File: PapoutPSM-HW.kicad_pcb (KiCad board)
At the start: 4 copper layers, 57 x 45 mm, 75 parts, among them J1 53015-0510, J2 53015-0510, Q1 NTK3134NT1G, Q2 NTK3134NT1G, Q3 NTK3134NT1G, U1 STM32G030F6, U2 SP3232EEY-L, U3 74HC4049, U4 TPS5430DDA, U5 RT8259GJ6

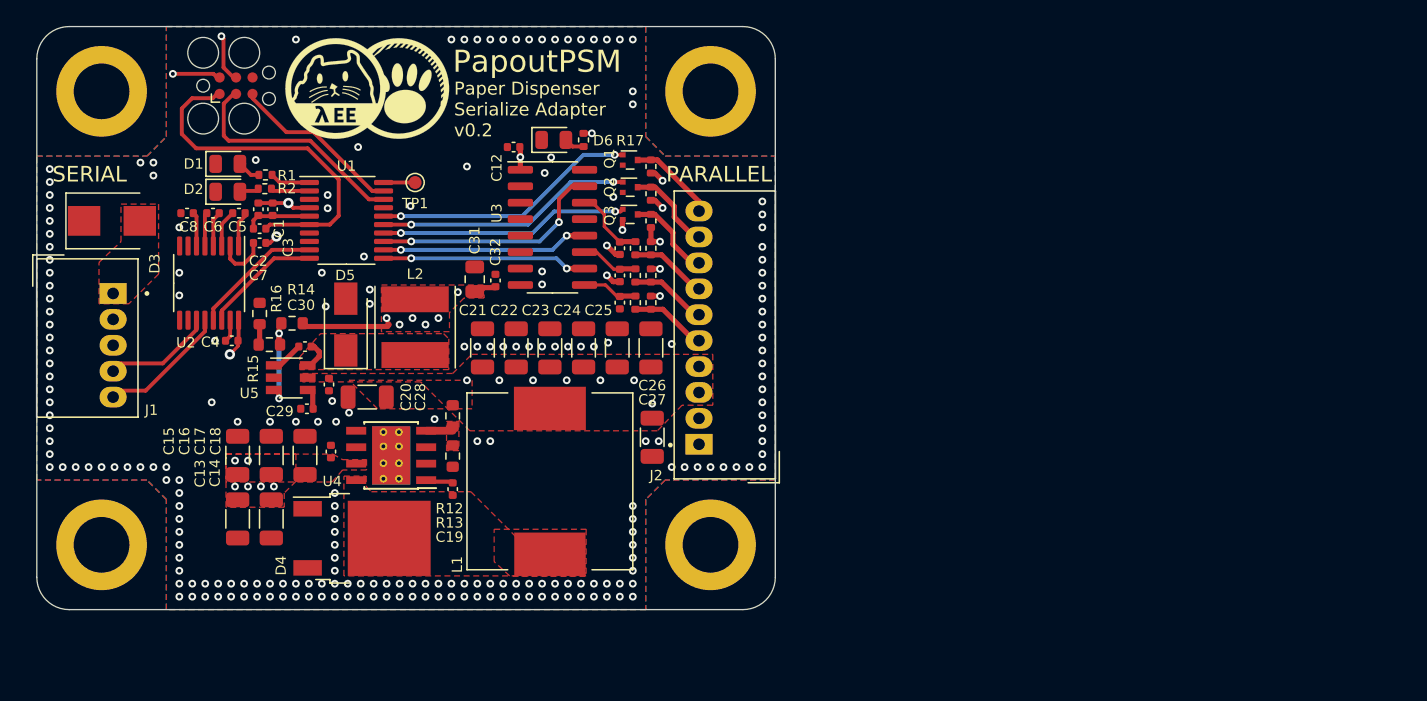
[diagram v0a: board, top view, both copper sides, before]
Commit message: release/v3 update
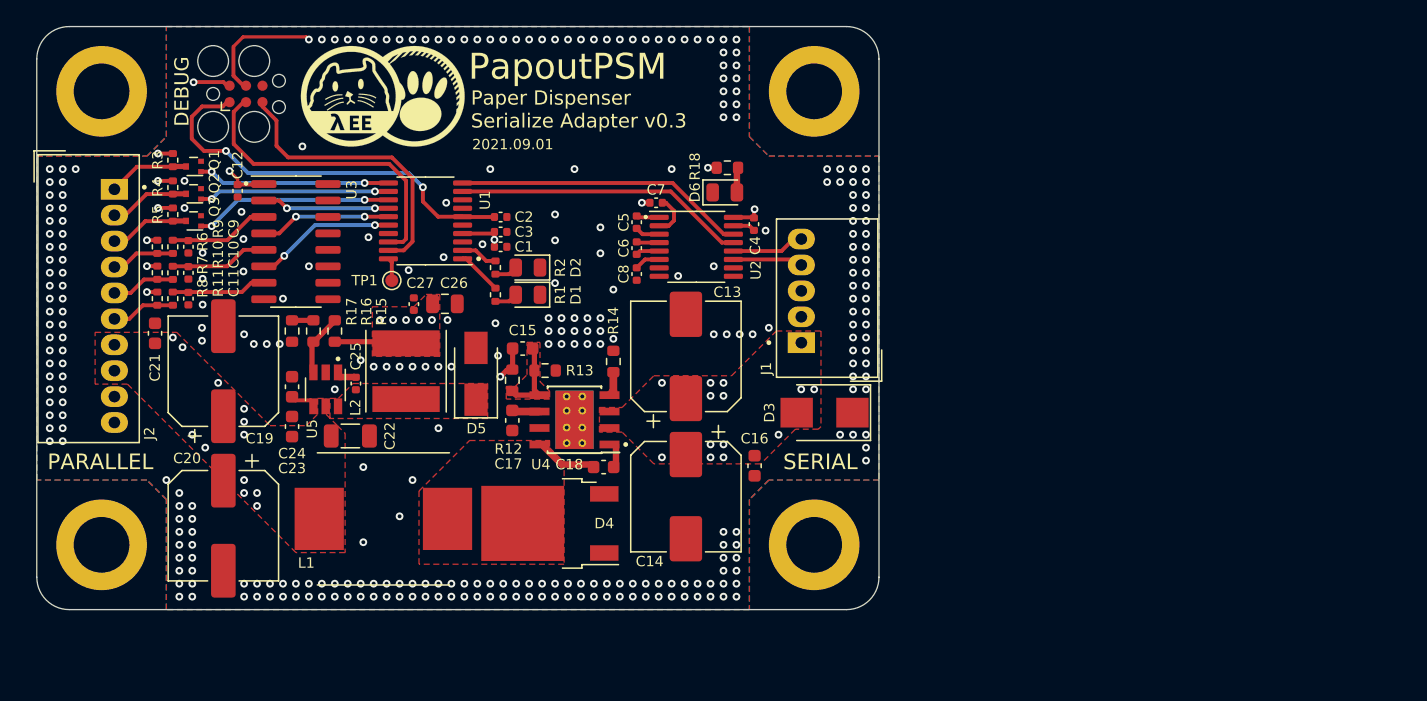
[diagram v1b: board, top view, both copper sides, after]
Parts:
- removed the C16 at (38.1, 83.1)
- removed the C22 at (57.0, 74.8)
- removed the C23 at (59.6, 74.8)
- removed the C24 at (62.2, 74.8)
- removed the C25 at (64.8, 74.8)
- removed the C26 at (67.4, 74.8)
- removed the C27 at (67.5, 81.7)
- added C19: 100uF, Capacitor_SMD:CP_Elec_8x6.9, F.Cu at (34.4, 76.6)
- added C20: 100uF, Capacitor_SMD:CP_Elec_8x6.9, F.Cu at (34.4, 88.5)
- added R14: 20k, Resistor_SMD:R_0603_1608Metric, F.Cu at (64.5, 75.8)
- C13, C14: value 10uF 50V -> 68uF; footprint Capacitor_SMD:C_1206_3216Metric -> Capacitor_SMD:CP_Elec_8x10
- C15: value 10uF 50V -> 330pF; footprint Capacitor_SMD:C_1206_3216Metric -> Capacitor_SMD:C_0603_1608Metric
- C16: renamed from C18; value 100nF -> 100nF 50V; footprint Capacitor_SMD:C_0402_1005Metric -> Capacitor_SMD:C_0603_1608Metric
- C17: value 10uF 50V -> 22nF; footprint Capacitor_SMD:C_1206_3216Metric -> Capacitor_SMD:C_0603_1608Metric
- C18: renamed from C19; value 10nF -> 100nF 50V; footprint Capacitor_SMD:C_0402_1005Metric -> Capacitor_SMD:C_0603_1608Metric
- C21: value 10uF 50V -> 100nF 50V; footprint Capacitor_SMD:C_1206_3216Metric -> Capacitor_SMD:C_0603_1608Metric
- C23: renamed from C20; value 100nF -> 100nF 50V; footprint Capacitor_SMD:C_0402_1005Metric -> Capacitor_SMD:C_0603_1608Metric
- C24: renamed from C29; value 100nF -> 100nF 50V; footprint Capacitor_SMD:C_0402_1005Metric -> Capacitor_SMD:C_0603_1608Metric
- D4: value MBRD20200CT-13 -> MBRD20150CT-13
- L1: value MWSA1206S-330MT -> SPM10040T-4R7M; footprint Power_Inductor_Extended:L_Sunlord-MWSA1206S -> TDK-SPM10040:L_TDK_SPM10040
- R12: renamed from R13; value 1.13k -> 150k
- R13: renamed from R12; value 10k -> 10k 0.1W
- R18: renamed from R17; value 4.7k -> 10k 0.1W; footprint Resistor_SMD:R_0402_1005Metric -> Resistor_SMD:R_0603_1608Metric
- R3, R4, R5: value 4.7k -> 8.2k
- R6, R7, R8: value 4.7k -> 27k
- U1: value STM32G030F6 -> STM32G031F8P6
- U4: value TPS5430DDA -> LMR14050SDDA
- moved H2 65.2 mm to (80.0, 90.0), turned to 90 degrees
- moved H4 65.2 mm to (80.0, 55.0), turned to 90 degrees
- moved H1 58.6 mm to (25.0, 90.0), turned to 90 degrees
- moved H3 58.6 mm to (25.0, 55.0), turned to 90 degrees
- moved D3 57.0 mm to (80.8, 79.8), turned to 180 degrees
- moved J1 53.3 mm to (79.0, 74.4), turned to 90 degrees
- moved J2 49.2 mm to (26.0, 62.6), turned to -90 degrees
- moved C4 41.3 mm to (75.3, 65.2), turned to -90 degrees
- moved R8 38.1 mm to (29.3, 71.0)
- moved R7 38.1 mm to (29.3, 69.0)
- moved R6 38.1 mm to (29.3, 67.0)
- moved U2 37.7 mm to (70.9, 67.0), turned to 0 degrees
- moved R3 36.9 mm to (30.5, 60.3), turned to 90 degrees
- moved R5 36.9 mm to (30.5, 64.5), turned to 90 degrees
- moved R4 36.9 mm to (30.5, 62.4), turned to 90 degrees
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- renumbered C28 to C22, C30 to C25, C31 to C26, C32 to C27, R14 to R15, R15 to R16, R16 to R17
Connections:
- net /Power/BIG_PH renamed /Power/BIG_SW
- net Net-(C19-Pad1) renamed /Power/BIG_BOOT
- C15 pad 1: +24V -> +12V
- C15 pad 2: GND -> /Power/BIG_FB
- C17 pad 1: +24V -> /Power/BIG_SS
- J2 pad 1: GND -> /Parallel_IO/J_INHIBIT
- J2 pad 10: /Parallel_IO/J_INHIBIT -> GND
- J2 pad 2: GND -> /Parallel_IO/J_RESET
- J2 pad 3: +12V -> /Parallel_IO/J_PULSE
- J2 pad 4: +12V -> /Parallel_IO/J_OUT_PULSE
- J2 pad 5: /Parallel_IO/J_ERROR -> /Parallel_IO/J_EMPTY
- J2 pad 6: /Parallel_IO/J_EMPTY -> /Parallel_IO/J_ERROR
- J2 pad 7: /Parallel_IO/J_OUT_PULSE -> +12V
- J2 pad 8: /Parallel_IO/J_PULSE -> +12V
- J2 pad 9: /Parallel_IO/J_RESET -> GND
- R12 pad 1: /Power/BIG_VS -> +12V
- R12 pad 2: GND -> /Power/BIG_FB
- R13 pad 1: +12V -> /Power/BIG_FB
- R13 pad 2: /Power/BIG_VS -> GND
- U1 pad 11: /P_ERROR -> /P_INHIBIT
- U1 pad 12: /P_EMPTY -> /P_RESET
- U1 pad 13: /P_OUT_PULSE -> /P_PULSE
- U1 pad 14: /P_PULSE -> /P_OUT_PULSE
- U1 pad 15: /P_RESET -> /P_EMPTY
- U1 pad 16: /P_INHIBIT -> /P_ERROR
- U3 pad 10: /P_ERROR -> unconnected-(U3-Pad10)
- U3 pad 11: Net-(C10-Pad1) -> GND
- U3 pad 12: /P_EMPTY -> unconnected-(U3-Pad12)
- U3 pad 14: Net-(C9-Pad1) -> GND
- U3 pad 15: /P_OUT_PULSE -> unconnected-(U3-Pad15)
- U3 pad 2: unconnected-(U3-Pad2) -> /P_OUT_PULSE
- U3 pad 3: GND -> Net-(C9-Pad1)
- U3 pad 4: unconnected-(U3-Pad4) -> /P_EMPTY
- U3 pad 5: GND -> Net-(C10-Pad1)
- U3 pad 6: unconnected-(U3-Pad6) -> /P_ERROR
- U3 pad 7: GND -> Net-(C11-Pad1)
- U3 pad 9: Net-(C11-Pad1) -> GND
- U4 pad 2: unconnected-(U4-Pad2) -> +24V
- U4 pad 3: unconnected-(U4-Pad3) -> +24V
- U4 pad 4: /Power/BIG_VS -> /Power/BIG_RTS
- U4 pad 5: unconnected-(U4-Pad5) -> /Power/BIG_FB
- U4 pad 6: GND -> /Power/BIG_SS
- U4 pad 7: +24V -> GND
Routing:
- net /M_RX: track 9.17 -> 22.5 mm
- net /M_TX: track 10.2 -> 22.5 mm
- net /SWCLK: track 13.6 -> 22.5 mm
- net /P_OUT_PULSE: track 18.3 -> 10.2 mm
- net /SWDIO: track 17.9 -> 24.0 mm
- net /Power/BIG_FB: track 0.00 -> 5.97 mm
- net /P_EMPTY: track 16.0 -> 10.4 mm
- net /P_INHIBIT: track 20.4 -> 15.1 mm
- net /Power/BIG_SW: track 0.00 -> 4.90 mm
- net /P_RESET: track 19.8 -> 15.0 mm
- net /P_ERROR: track 15.8 -> 11.2 mm
- net /R_RXD: track 10.0 -> 5.63 mm
- net +3V3: track 23.1 -> 19.0 mm, vias 12 -> 11
- net /NRST: track 27.5 -> 31.4 mm, vias 0 -> 2
- net /P_PULSE: track 19.2 -> 15.6 mm
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- added copper zone on F.Cu, net /Power/BIG_FB
- removed copper zone on F.Cu, net /Power/BIG_VS
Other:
- board size 57 x 45 mm -> 65 x 45 mm
- board text added: "2021.09.01"
- board text added: "DEBUG"
- board text added: "Paper Dispenser Serialize Adapter v0.3"
- board text added: "github.com/pmnxis/PapoutPSM-HW CERN-OHL-S-2.0"
- board text removed: "Paper Dispenser Serialize Adapter v0.2"
- board text removed: "github.com/PapoutPSM-HW CERN-OHL-S-2.0"

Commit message: before release v0.5
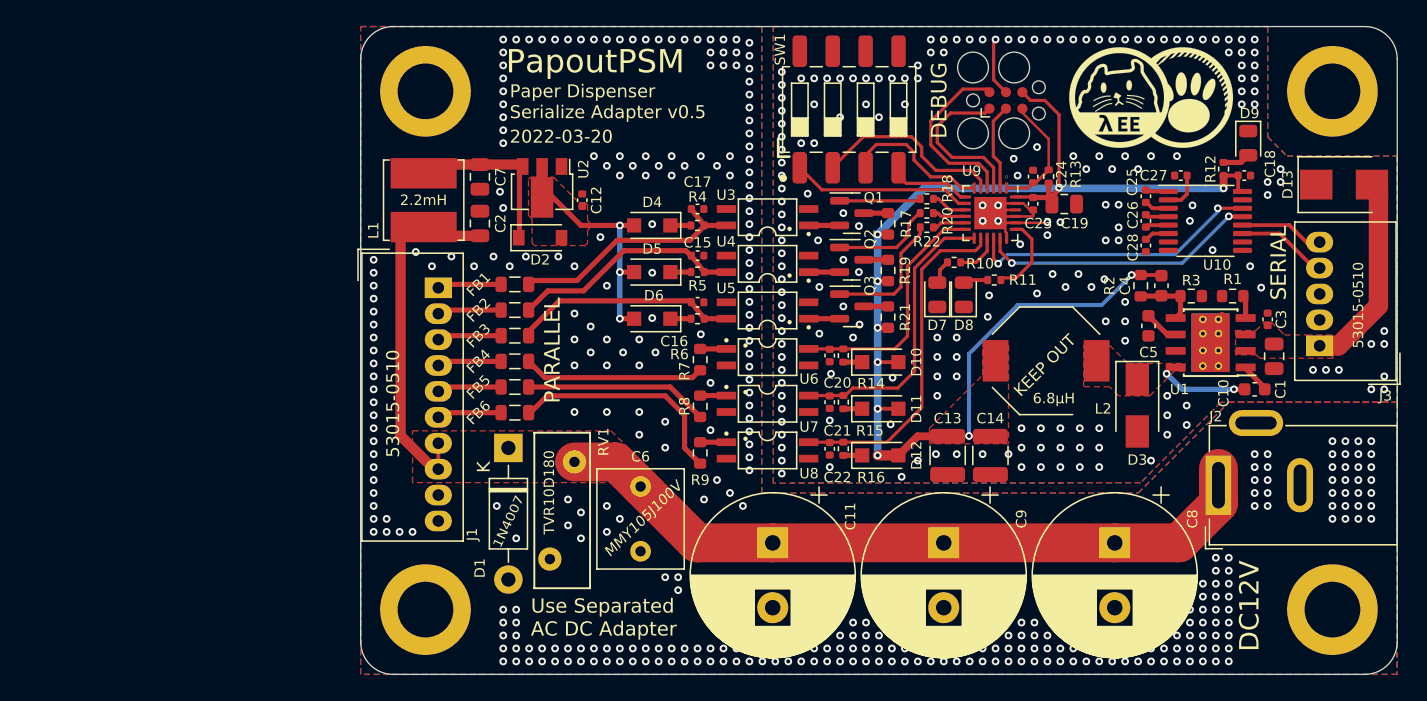
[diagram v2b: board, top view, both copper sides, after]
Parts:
- removed TP1: TestPoint, TestPoint:TestPoint_Pad_D1.0mm
- added C28: 100nF, Capacitor_SMD:C_0402_1005Metric, F.Cu at (105.6, 66.9)
- added D10: 1N4007, Diode_SMD:D_SOD-123F, F.Cu at (85.1, 75.9)
- added D11: 1N4007, Diode_SMD:D_SOD-123F, F.Cu at (85.1, 79.5)
- added D12: 1N4007, Diode_SMD:D_SOD-123F, F.Cu at (85.1, 83.1)
- added D13: SMBJ28CA, Diode_SMD:D_SMB, F.Cu at (120.9, 62.2)
- added D7: LED_YELLOW, LED_SMD:LED_0805_2012Metric, F.Cu at (89.5, 70.7)
- added D8: LED_YELLOW, LED_SMD:LED_0805_2012Metric, F.Cu at (91.5, 70.7)
- added D9: LED GREEN, LED_SMD:LED_0805_2012Metric, F.Cu at (113.5, 59.0)
- added FB1: GZ2012D601TF, Inductor_SMD:L_0805_2012Metric, F.Cu at (56.9, 69.9)
- added FB2: GZ2012D601TF, Inductor_SMD:L_0805_2012Metric, F.Cu at (56.9, 71.9)
- added FB3: GZ2012D601TF, Inductor_SMD:L_0805_2012Metric, F.Cu at (56.9, 73.9)
- added FB4: GZ2012D601TF, Inductor_SMD:L_0805_2012Metric, F.Cu at (56.9, 75.8)
- added FB5: GZ2012D601TF, Inductor_SMD:L_0805_2012Metric, F.Cu at (56.9, 77.8)
- added FB6: GZ2012D601TF, Inductor_SMD:L_0805_2012Metric, F.Cu at (56.9, 79.8)
- added J3: 53015-0510, Molex-53015:Molex_MicroBlade_53015-0500_1x05_P2.00mm_Right, F.Cu at (119.0, 74.6)
- added R19: 660, Resistor_SMD:R_0603_1608Metric, F.Cu at (85.7, 68.8)
- added R20: 4.7k, Resistor_SMD:R_0402_1005Metric, F.Cu at (88.7, 64.4)
- added R21: 660, Resistor_SMD:R_0603_1608Metric, F.Cu at (85.7, 72.4)
- added R22: 4.7k, Resistor_SMD:R_0402_1005Metric, F.Cu at (88.7, 65.5)
- added RV1: 10Ø 18V, Varistor:RV_Disc_D12mm_W4.3mm_P7.5mm, F.Cu at (61.5, 83.6)
- added SW1: DSIC04LSGET, Button_Switch_SMD_Extended:SW_DIP_SPSTx04_Slide_9.30x10.16mm_W4.25mm_P2.54mm, F.Cu at (82.7, 56.4)
- added U10: SP3232EEY-L, Package_SO:TSSOP-16_4.4x5mm_P0.65mm, F.Cu at (110.2, 65.0)
- added U6: EL3H7-G, EL3H7-G:SMDIP-4_W5.20mm, F.Cu at (76.4, 75.5)
- added U7: EL3H7-G, EL3H7-G:SMDIP-4_W5.20mm, F.Cu at (76.4, 79.1)
- added U8: EL3H7-G, EL3H7-G:SMDIP-4_W5.20mm, F.Cu at (76.4, 82.7)
- added U9: MSP430FR2433IRGE, Package_DFN_QFN:HVQFN-24-1EP_4x4mm_P0.5mm_EP2.5x2.5mm, F.Cu at (93.6, 64.4)
- C1: value 4.7uF -> 10uF 50V; footprint Capacitor_SMD:C_0402_1005Metric -> Capacitor_SMD:C_0805_2012Metric
- C10: value 10nF -> 100nF 50V; footprint Capacitor_SMD:C_0402_1005Metric -> Capacitor_SMD:C_0603_1608Metric
- C11, C9: value 10nF -> 1.8mF; footprint Capacitor_SMD:C_0402_1005Metric -> Capacitor_THT:CP_Radial_D12.5mm_P5.00mm
- C13, C14: value 68uF -> 47uF; footprint Capacitor_SMD:CP_Elec_8x10 -> Capacitor_SMD:C_1210_3225Metric
- C15: value 330pF -> 100nF; footprint Capacitor_SMD:C_0603_1608Metric -> Capacitor_SMD:C_0402_1005Metric
- C16, C18, C21, C23: value 100nF 50V -> 100nF; footprint Capacitor_SMD:C_0603_1608Metric -> Capacitor_SMD:C_0402_1005Metric
- C17: value 22nF -> 100nF; footprint Capacitor_SMD:C_0603_1608Metric -> Capacitor_SMD:C_0402_1005Metric
- C19: value 100uF -> 10uF 50V; footprint Capacitor_SMD:CP_Elec_8x6.9 -> Capacitor_SMD:C_0805_2012Metric
- C2, C7: value 100nF -> 330nF; footprint Capacitor_SMD:C_0402_1005Metric -> Capacitor_SMD:C_0805_2012Metric
- C20: value 100uF -> 100nF; footprint Capacitor_SMD:CP_Elec_8x6.9 -> Capacitor_SMD:C_0402_1005Metric
- C22: value 10uF 50V -> 100nF; footprint Capacitor_SMD:C_1206_3216Metric -> Capacitor_SMD:C_0402_1005Metric
- C24: value 100nF 50V -> 1nF; footprint Capacitor_SMD:C_0603_1608Metric -> Capacitor_SMD:C_0402_1005Metric
- C25: value 10nF -> 100nF
- C26: value 22uF -> 100nF; footprint Capacitor_SMD:C_0805_2012Metric -> Capacitor_SMD:C_0402_1005Metric
- C4: value 100nF -> 220pF; footprint Capacitor_SMD:C_0402_1005Metric -> Capacitor_SMD:C_0603_1608Metric
- C5: value 100nF -> 22nF; footprint Capacitor_SMD:C_0402_1005Metric -> Capacitor_SMD:C_0603_1608Metric
- C6: value 100nF -> 1uF; footprint Capacitor_SMD:C_0402_1005Metric -> Capacitor_THT:C_Rect_L7.5mm_W6.5mm_P5.00mm
- C8: value 100nF -> 1.8mF; footprint Capacitor_SMD:C_0402_1005Metric -> Capacitor_THT:CP_Radial_D12.5mm_P5.00mm
- D1: value LED_YELLOW -> 1N4007; footprint LED_SMD:LED_0805_2012Metric -> Diode_THT:D_DO-41_SOD81_P10.16mm_Horizontal
- D2: value LED_YELLOW -> 1N4148W; footprint LED_SMD:LED_0805_2012Metric -> Diode_SMD:D_SOD-123
- D3: value SMBJ28CA -> SS34; footprint Diode_SMD:D_SMB -> Diode_SMD:D_SMA
- D4: value MBRD20150CT-13 -> 1N4007; footprint Package_TO_SOT_SMD:TO-252-2 -> Diode_SMD:D_SOD-123F
- D5: value B240AQ-13-F -> 1N4007; footprint Diode_SMD:D_SMA -> Diode_SMD:D_SOD-123F
- D6: value LED GREEN -> 1N4007; footprint LED_SMD:LED_0805_2012Metric -> Diode_SMD:D_SOD-123F
- J1: footprint Molex-53015:Molex_MicroBlade_53015-0500_1x05_P2.00mm_Right -> Molex-53015:Molex_MicroBlade_53015-1000_1x10_P2.00mm_Right
- J2: value 53015-0510 -> Barrel_Jack; footprint Molex-53015:Molex_MicroBlade_53015-1000_1x10_P2.00mm_Right -> Connector_BarrelJack:BarrelJack_GCT_DCJ200-10-A_Horizontal
- L1: value SPM10040T-4R7M -> FNR6045S222KT; footprint TDK-SPM10040:L_TDK_SPM10040 -> Inductor_SMD:L_Bourns_SRN6045TA
- L2: value VLS6045EX-4R7M -> CDRH8D43NP-6R8NC; footprint Power_Inductor_Extended:L_TDK_VLS6045EX -> Inductor_SMD:L_Bourns-SRU8028_8.0x8.0mm
- Q1, Q2, Q3: value NTK3134NT1G -> 2N7002; footprint Package_TO_SOT_SMD:SOT-723 -> Package_TO_SOT_SMD:SOT-23
- R1: value 4.7k -> 20k; footprint Resistor_SMD:R_0402_1005Metric -> Resistor_SMD:R_0603_1608Metric
- R10, R11: value 51k -> 4.7k
- R12: value 150k -> 10k; footprint Resistor_SMD:R_0603_1608Metric -> Resistor_SMD:R_0402_1005Metric
- R13: value 10k 0.1W -> 47k; footprint Resistor_SMD:R_0603_1608Metric -> Resistor_SMD:R_0402_1005Metric
- R14: value 20k -> 4.7k; footprint Resistor_SMD:R_0603_1608Metric -> Resistor_SMD:R_0402_1005Metric
- R15: value 62k -> 4.7k; footprint Resistor_SMD:R_0603_1608Metric -> Resistor_SMD:R_0402_1005Metric
- R16: value 16k -> 4.7k; footprint Resistor_SMD:R_0603_1608Metric -> Resistor_SMD:R_0402_1005Metric
- R17: value 3.6k -> 660
- R18: value 10k 0.1W -> 4.7k; footprint Resistor_SMD:R_0603_1608Metric -> Resistor_SMD:R_0402_1005Metric
- R2: value 4.7k -> 68k; footprint Resistor_SMD:R_0402_1005Metric -> Resistor_SMD:R_0603_1608Metric
- R3: value 8.2k -> 12k; footprint Resistor_SMD:R_0402_1005Metric -> Resistor_SMD:R_0603_1608Metric
- R4, R5: value 8.2k -> 4.7k
- R6: value 27k -> 4.7k
- R7, R8: value 27k -> 330; footprint Resistor_SMD:R_0402_1005Metric -> Resistor_SMD:R_0603_1608Metric
- R9: value 51k -> 330; footprint Resistor_SMD:R_0402_1005Metric -> Resistor_SMD:R_0603_1608Metric
- U1: value STM32G031F8P6 -> LMR14020SDDA; footprint Package_SO:TSSOP-20_4.4x6.5mm_P0.65mm -> Package_SO:TI_SO-PowerPAD-8_ThermalVias
- U2: value SP3232EEY-L -> 78L05G-AB3-R; footprint Package_SO:TSSOP-16_4.4x5mm_P0.65mm -> Package_TO_SOT_SMD:SOT-89-3
- U3: value 74HC4049 -> EL3H7-G; footprint Package_SO:SOIC-16_3.9x9.9mm_P1.27mm -> EL3H7-G:SMDIP-4_W5.20mm
- U4: value LMR14050SDDA -> EL3H7-G; footprint Package_SO:TI_SO-PowerPAD-8_ThermalVias -> EL3H7-G:SMDIP-4_W5.20mm
- U5: value RT8259GJ6 -> EL3H7-G; footprint Package_TO_SOT_SMD:TSOT-23-6 -> EL3H7-G:SMDIP-4_W5.20mm
- moved H1 95.1 mm to (120.0, 95.0), turned to 180 degrees
- moved H3 95.0 mm to (120.0, 55.0), turned to 180 degrees
- moved J2 88.2 mm to (111.2, 85.4), turned to 90 degrees
- moved C10 82.8 mm to (114.0, 78.0), turned to 180 degrees
- moved R3 79.3 mm to (109.1, 70.8), turned to 0 degrees
- moved C19 66.2 mm to (99.3, 63.7), turned to 0 degrees
- moved R11 63.4 mm to (93.9, 69.6), turned to 180 degrees
- moved C25 62.7 mm to (105.6, 63.1), turned to 90 degrees
- moved C9 62.6 mm to (90.0, 89.8)
- moved U1 61.3 mm to (110.6, 74.4)
- moved R10 60.3 mm to (90.8, 68.2), turned to 180 degrees
- moved C1 60.3 mm to (115.5, 75.5), turned to -90 degrees
- moved C27 60.0 mm to (108.3, 61.5), turned to 0 degrees
- moved C23 59.7 mm to (96.9, 63.7), turned to -90 degrees
- moved C3 59.6 mm to (115.0, 72.6), turned to 90 degrees
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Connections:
- C1 pad 1: +3V3 -> +24V
- C10 pad 1: Net-(C10-Pad1) -> /BIG_BOOT
- C10 pad 2: GND -> /BIG_SW
- C11 pad 1: Net-(C11-Pad1) -> +12VA
- C11 pad 2: GND -> GNDA
- C12 pad 1: +3V3 -> +5VA
- C12 pad 2: GND -> GNDA
- C13 pad 1: +24V -> +3V3
- C14 pad 1: +24V -> +3V3
- C15 pad 1: +12V -> GNDA
- C15 pad 2: /Power/BIG_FB -> /J_RESET
- C16 pad 1: +24V -> GNDA
- C16 pad 2: GND -> /J_PULSE
- C17 pad 1: /Power/BIG_SS -> GNDA
- C17 pad 2: GND -> /J_INHIBIT
- C18 pad 1: /Power/BIG_BOOT -> +3V3
- C18 pad 2: /Power/BIG_SW -> GND
- C19 pad 1: +12V -> +3V3
- C2 pad 1: /NRST -> +12VA
- C2 pad 2: GND -> GNDA
- C20 pad 1: +12V -> /P_OUT_PULSE
- C21 pad 1: +12V -> /P_EMPTY
- C22 pad 1: +12V -> /P_ERROR
- C23 pad 1: +12V -> +3V3
- C24 pad 1: /Power/PWR_EN -> /NRST
- C25 pad 1: /Power/PWR_BOOT -> Net-(C25-Pad1)
- C25 pad 2: /Power/PWR_PHASE -> Net-(C25-Pad2)
- C26 pad 1: +3V3 -> Net-(C26-Pad1)
- C26 pad 2: GND -> Net-(C26-Pad2)
- C27 pad 1: +3V3 -> GND
- C27 pad 2: GND -> Net-(C27-Pad2)
- C3 pad 1: +3V3 -> +24V
- C4 pad 2: GND -> /BIG_FB
- C5 pad 1: Net-(C5-Pad1) -> /BIG_SS
- C5 pad 2: Net-(C5-Pad2) -> GND
- C6 pad 1: Net-(C6-Pad1) -> +12VA
- C6 pad 2: Net-(C6-Pad2) -> GNDA
- C7 pad 1: Net-(C7-Pad1) -> /+FILTERED_12VA
- C7 pad 2: +3V3 -> GNDA
- C8 pad 1: Net-(C8-Pad1) -> +12VA
- C8 pad 2: GND -> GNDA
- C9 pad 1: Net-(C9-Pad1) -> +12VA
- C9 pad 2: GND -> GNDA
- D1 pad 1: GND -> +12VA
- D1 pad 2: Net-(D1-Pad2) -> GNDA
- D2 pad 1: GND -> /+FILTERED_12VA
- D2 pad 2: Net-(D2-Pad2) -> +5VA
- D3 pad 1: GND -> /BIG_SW
- D3 pad 2: +24V -> GND
- D4 pad 1: GND -> Net-(D4-Pad1)
- D4 pad 2: /Power/BIG_SW -> +5VA
- D5 pad 1: /Power/PWR_PHASE -> Net-(D5-Pad1)
- D5 pad 2: GND -> +5VA
- D6 pad 1: GND -> Net-(D6-Pad1)
- D6 pad 2: Net-(D6-Pad2) -> +5VA
- DEBUG1 pad 1: /NRST -> /D_TX
- DEBUG1 pad 2: +3V3 -> /D_RX
- DEBUG1 pad 3: /SWDIO -> /TEST
- DEBUG1 pad 5: /SWCLK -> /NRST
- DEBUG1 pad 6: unconnected-(DEBUG1-Pad6) -> +3V3
- J1 pad 1: +24V -> /EX_INHIBIT
- J1 pad 2: GND -> /EX_RESET
- J1 pad 3: GND -> /EX_PULSE
- J1 pad 4: /R_TXD -> /EX_OUT_PULSE
- J1 pad 5: /R_RXD -> /EX_EMPTY
- J2 pad 1: /Parallel_IO/J_INHIBIT -> +12VA
- J2 pad 2: /Parallel_IO/J_RESET -> GNDA
- J2 pad 3: /Parallel_IO/J_PULSE -> GNDA
- L1 pad 1: /Power/BIG_SW -> +12VA
- L1 pad 2: +12V -> /+FILTERED_12VA
- L2 pad 1: /Power/PWR_PHASE -> /BIG_SW
- Q1 pad 1: /P_INHIBIT -> Net-(Q1-Pad1)
- Q1 pad 2: GND -> /ANODE_INHIBIT
- Q1 pad 3: /Parallel_IO/J_INHIBIT -> Net-(Q1-Pad3)
- Q2 pad 1: /P_RESET -> Net-(Q2-Pad1)
- Q2 pad 2: GND -> /ANODE_RESET
- Q2 pad 3: /Parallel_IO/J_RESET -> Net-(Q2-Pad3)
- Q3 pad 1: /P_PULSE -> Net-(Q3-Pad1)
- Q3 pad 2: GND -> /ANODE_PULSE
- Q3 pad 3: /Parallel_IO/J_PULSE -> Net-(Q3-Pad3)
- R1 pad 1: /LED0 -> /BIG_RTS
- R1 pad 2: Net-(D1-Pad2) -> GND
- R10 pad 1: /Parallel_IO/J_EMPTY -> /LED0
- R10 pad 2: Net-(C10-Pad1) -> Net-(D7-Pad2)
- R11 pad 1: /Parallel_IO/J_ERROR -> /LED1
- R11 pad 2: Net-(C11-Pad1) -> Net-(D8-Pad2)
- R12 pad 1: +12V -> +3V3
- R12 pad 2: /Power/BIG_FB -> Net-(D9-Pad2)
- R13 pad 1: /Power/BIG_FB -> /NRST
- R13 pad 2: GND -> +3V3
- R14 pad 1: /Power/BIG_RTS -> Net-(D10-Pad1)
- R14 pad 2: GND -> /P_OUT_PULSE
- R15 pad 1: +3V3 -> Net-(D11-Pad1)
- R15 pad 2: /Power/PWR_FB -> /P_EMPTY
- R16 pad 1: /Power/PWR_FB -> Net-(D12-Pad1)
- R16 pad 2: Net-(R16-Pad2) -> /P_ERROR
- R17 pad 1: Net-(R16-Pad2) -> Net-(Q1-Pad3)
- R17 pad 2: GND -> +3V3
- R18 pad 1: +3V3 -> Net-(Q1-Pad1)
- R18 pad 2: Net-(D6-Pad2) -> /P_INHIBIT
- R2 pad 1: /LED1 -> +3V3
- R2 pad 2: Net-(D2-Pad2) -> /BIG_FB
- R3 pad 1: /Parallel_IO/J_INHIBIT -> /BIG_FB
- R3 pad 2: +12V -> GND
- R4 pad 1: /Parallel_IO/J_RESET -> Net-(D4-Pad1)
- R4 pad 2: +12V -> /J_INHIBIT
- R5 pad 1: /Parallel_IO/J_PULSE -> Net-(D5-Pad1)
- R5 pad 2: +12V -> /J_RESET
- R6 pad 1: /Parallel_IO/J_OUT_PULSE -> Net-(D6-Pad1)
- R6 pad 2: +12V -> /J_PULSE
- R7 pad 1: /Parallel_IO/J_EMPTY -> /J_OUT_PULSE
- R7 pad 2: +12V -> /ANODE_OUT_PULSE
- R8 pad 1: /Parallel_IO/J_ERROR -> /J_EMPTY
- R8 pad 2: +12V -> /ANODE_EMPTY
- R9 pad 1: /Parallel_IO/J_OUT_PULSE -> /J_ERROR
- R9 pad 2: Net-(C9-Pad1) -> /ANODE_ERROR
- U1 pad 1: /LED0 -> /BIG_BOOT
- U1 pad 2: /LED1 -> +24V
- U1 pad 3: GND -> +24V
- U1 pad 4: +3V3 -> /BIG_RTS
- U1 pad 5: GND -> /BIG_FB
- U1 pad 6: /NRST -> /BIG_SS
- U1 pad 8: GND -> /BIG_SW
- U1 pad 9: /M_TX -> GND
- U2 pad 1: Net-(C5-Pad2) -> GNDA
- U2 pad 2: Net-(C7-Pad1) -> +5VA
- U2 pad 3: Net-(C5-Pad1) -> /+FILTERED_12VA
- U3 pad 1: +3V3 -> /ANODE_INHIBIT
- U3 pad 2: /P_OUT_PULSE -> GND
- U3 pad 3: Net-(C9-Pad1) -> GNDA
- U3 pad 4: /P_EMPTY -> /J_INHIBIT
- U4 pad 1: /Power/BIG_BOOT -> /ANODE_RESET
- U4 pad 2: +24V -> GND
- U4 pad 3: +24V -> GNDA
- U4 pad 4: /Power/BIG_RTS -> /J_RESET
- U5 pad 1: /Power/PWR_BOOT -> /ANODE_PULSE
- U5 pad 3: /Power/PWR_FB -> GNDA
- U5 pad 4: /Power/PWR_EN -> /J_PULSE
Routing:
- net +12VA: track 0.00 -> 84.6 mm
- net +3V3: track 19.0 -> 98.9 mm, vias 11 -> 10
- net /SWDIO: track 24.0 -> 0.00 mm
- net /SWCLK: track 22.5 -> 0.00 mm
- net /NRST: track 31.4 -> 9.30 mm, vias 2 -> 0
- net +5VA: track 0.00 -> 19.2 mm, vias 0 -> 3
- net /J_INHIBIT: track 0.00 -> 18.8 mm
- net /J_RESET: track 0.00 -> 17.9 mm
- net /J_ERROR: track 0.00 -> 17.4 mm
- net /J_PULSE: track 0.00 -> 17.2 mm
- net +24V: track 0.00 -> 15.4 mm, vias 13 -> 0
- net /P_ERROR: track 11.2 -> 26.5 mm, vias 2 -> 0
- net /SW1: track 0.00 -> 14.8 mm
- net /J_EMPTY: track 0.00 -> 14.2 mm
- net /J_OUT_PULSE: track 0.00 -> 14.0 mm
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- added copper zone on F.Cu, net +12VA
- added copper zone on F.Cu, net +5VA
- added copper zone on F.Cu, net /BIG_SW
- added copper zone on B.Cu, net GNDA
- added copper zone on F.Cu, net GNDA
- removed copper zone on F.Cu, net +12V
- removed copper zone on In2.Cu, net +12V
- removed copper zone on In2.Cu, net +24V
- removed copper zone on In2.Cu, net +3V3
- removed copper zone on F.Cu, net /Power/BIG_FB
- removed copper zone on F.Cu, net /Power/BIG_SW
- removed copper zone on F.Cu, net /Power/PWR_PHASE
- removed copper zone on In1.Cu, net GND
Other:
- board size 65 x 45 mm -> 80 x 50 mm
- copper layers 4 -> 2
- board text added: "2.2mH"
- board text added: "2022-03-20"
- board text added: "6.8µH"
- board text added: "DC12V"
- board text added: "KEEP OUT"
- board text added: "Paper Dispenser Serialize Adapter v0.5"
- board text added: "Use Separated AC DC Adapter"
- board text removed: "2021.09.01"
- board text removed: "Paper Dispenser Serialize Adapter v0.3"
